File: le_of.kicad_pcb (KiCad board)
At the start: 4 copper layers, 19 parts, among them IC1 LTC3631EMS8E-3.3#PBF, IC2 STM32G0B1RET6N, J1 ST_Link_Connector

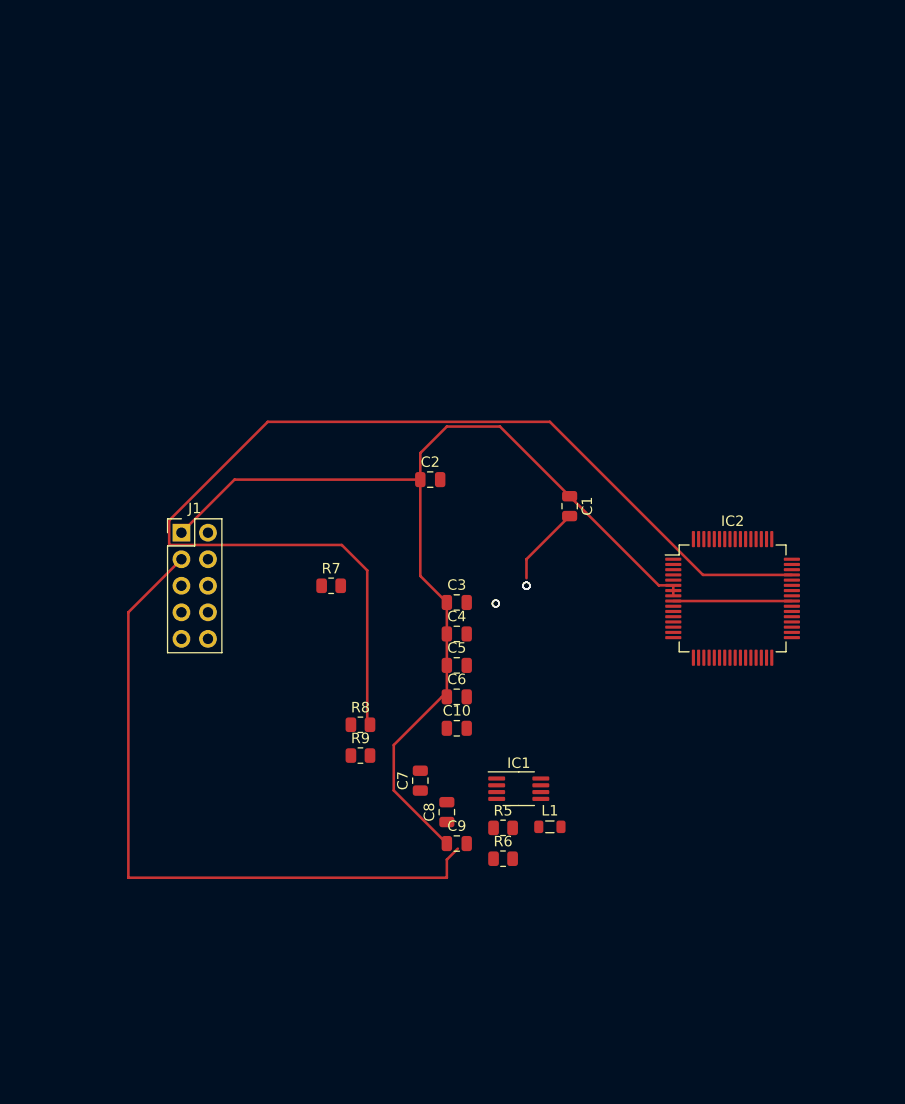
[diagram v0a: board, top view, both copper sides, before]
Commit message: made small changes
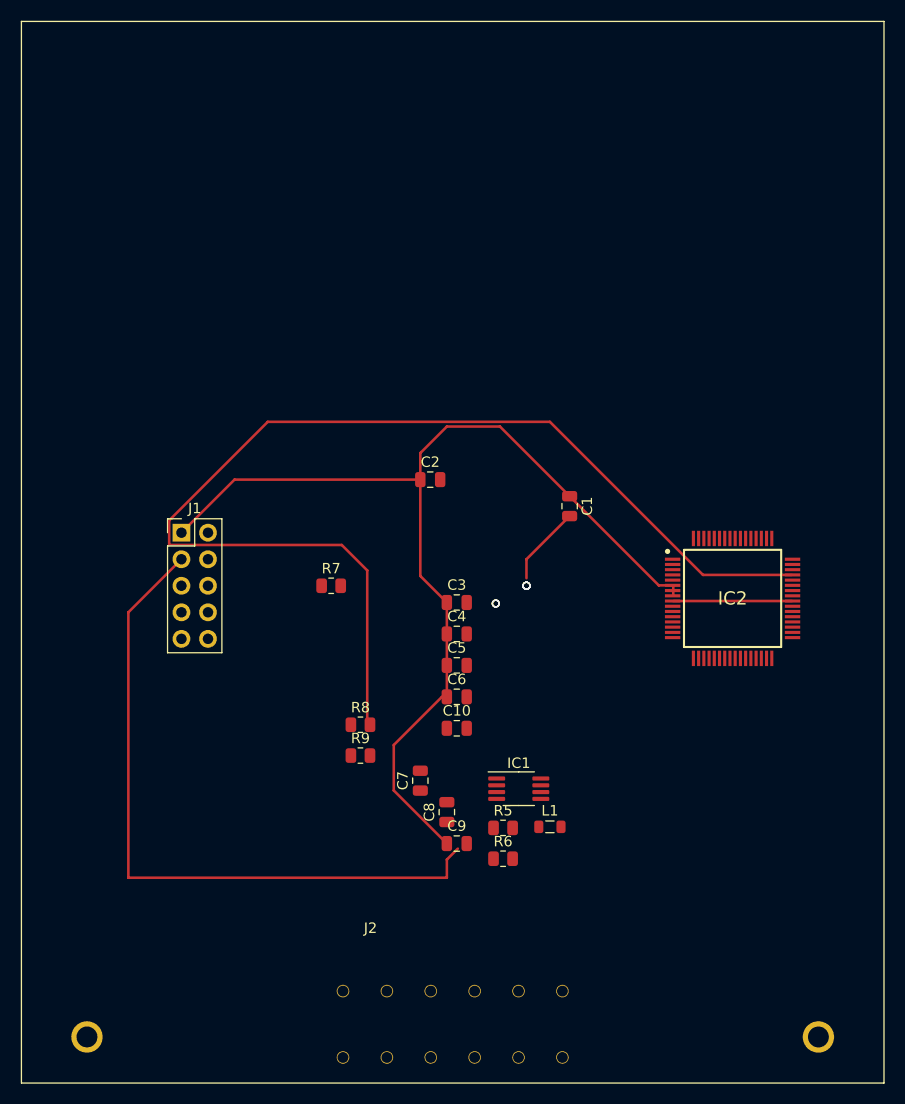
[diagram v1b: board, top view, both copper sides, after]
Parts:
- added J2: ATM13-12PA-R008, ATM13:ATM13-12PA-R008, F.Cu at (122.5, 111.1)
- IC2: footprint Package_QFP:LQFP-64_10x10mm_P0.5mm -> Sama:QFP50P1200X1200X160-64N
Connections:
- net Net-(J1-Pin_10) renamed /NSRT
- net Net-(J1-Pin_2) renamed /SWDIO
- net Net-(J1-Pin_4) renamed /SWCLK
